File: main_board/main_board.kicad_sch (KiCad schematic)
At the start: 10 parts

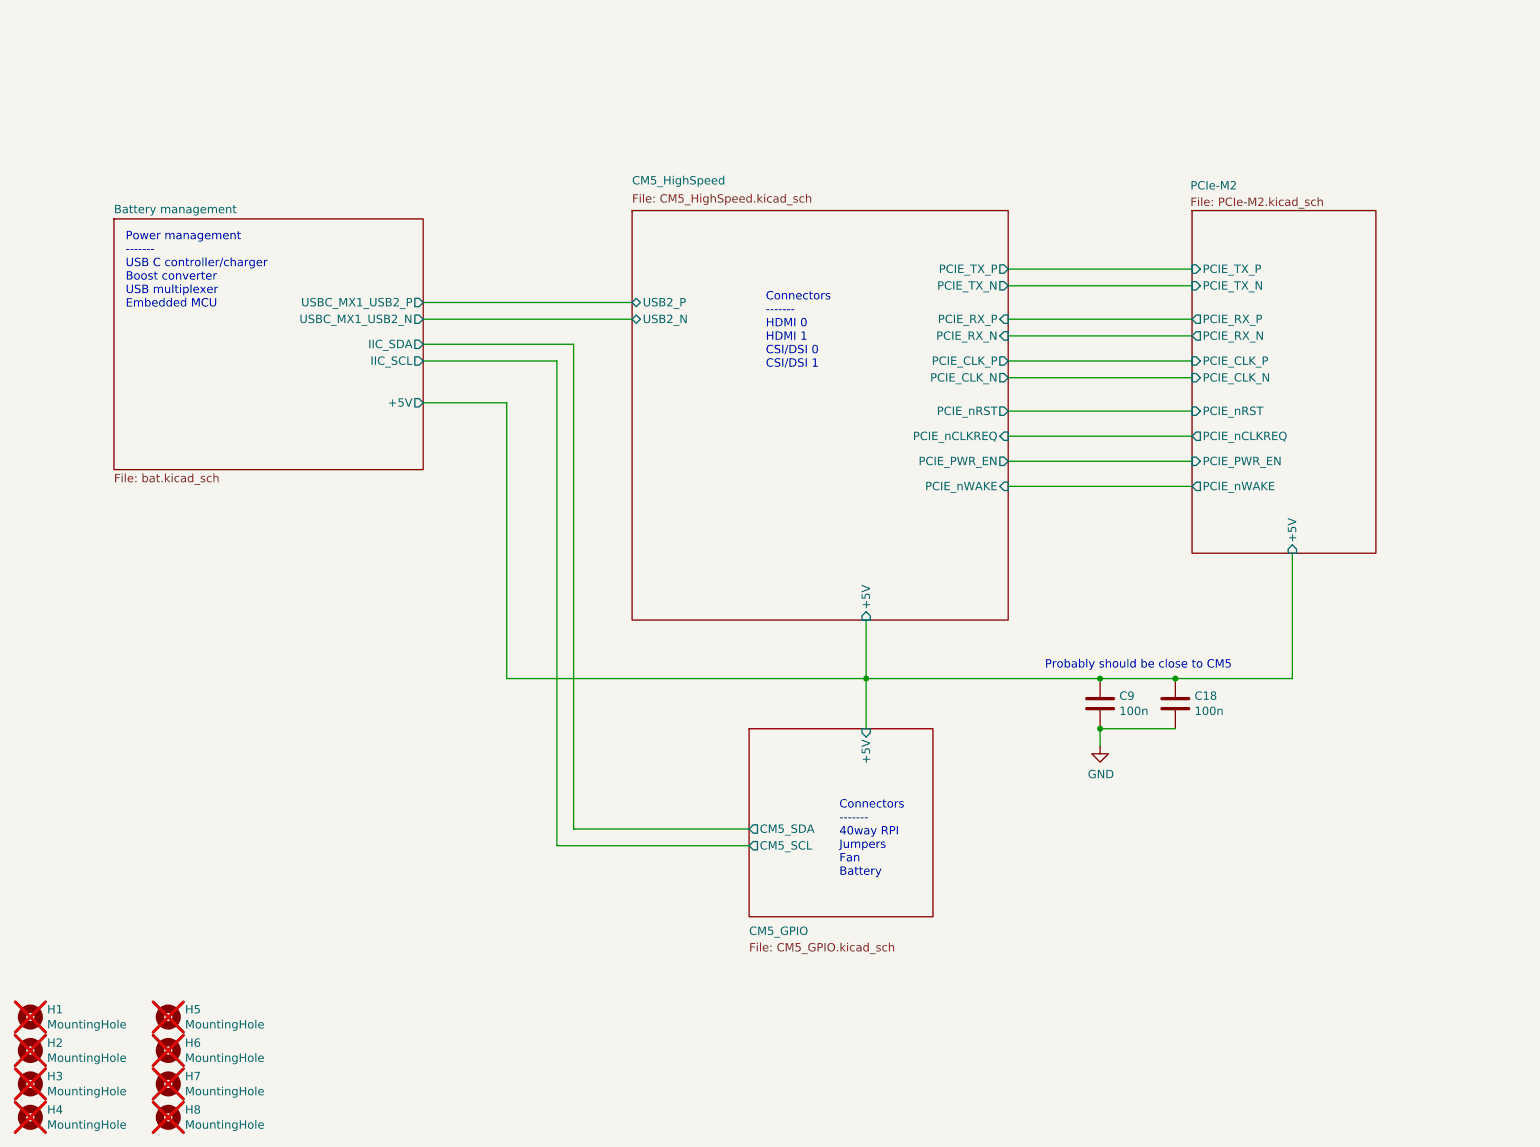
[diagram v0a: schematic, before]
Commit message: Finalize power management
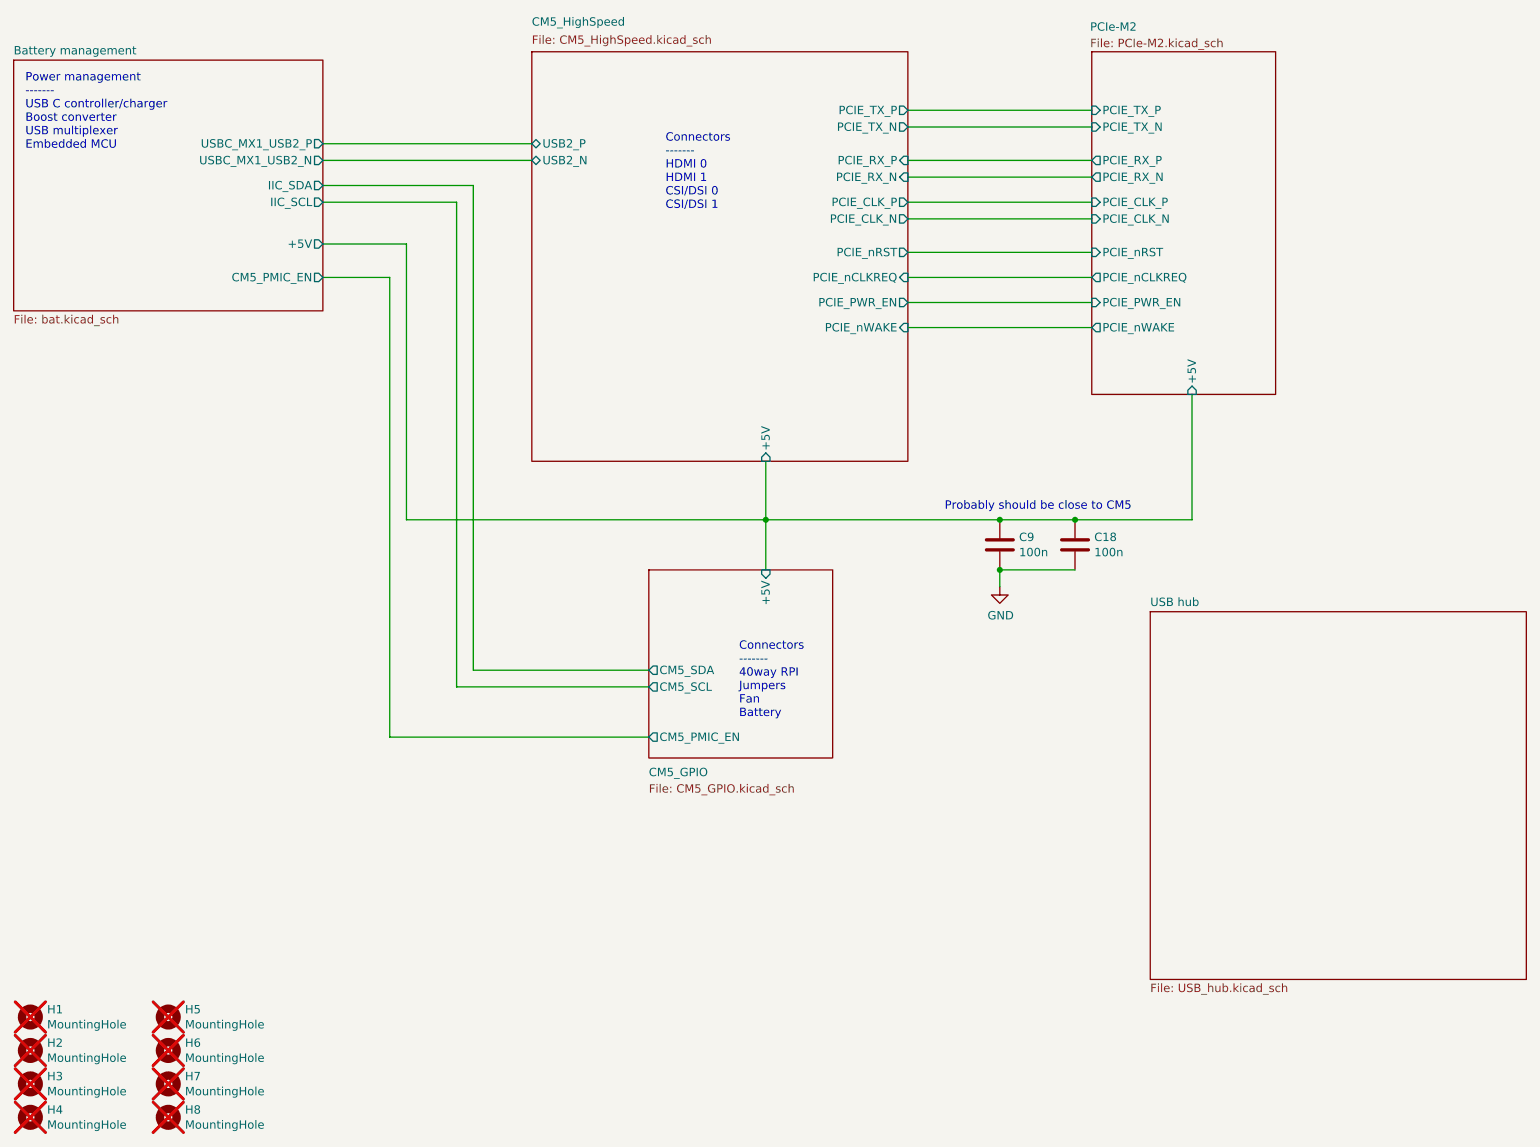
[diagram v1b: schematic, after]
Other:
- added sheet USB hub (USB_hub.kicad_sch)
- sheet Battery management ports: added CM5_PMIC_EN; removed none
- sheet CM5_GPIO ports: added CM5_PMIC_EN; removed none
- moved on the sheet: C18, C9
